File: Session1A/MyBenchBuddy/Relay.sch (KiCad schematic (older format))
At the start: 0 parts

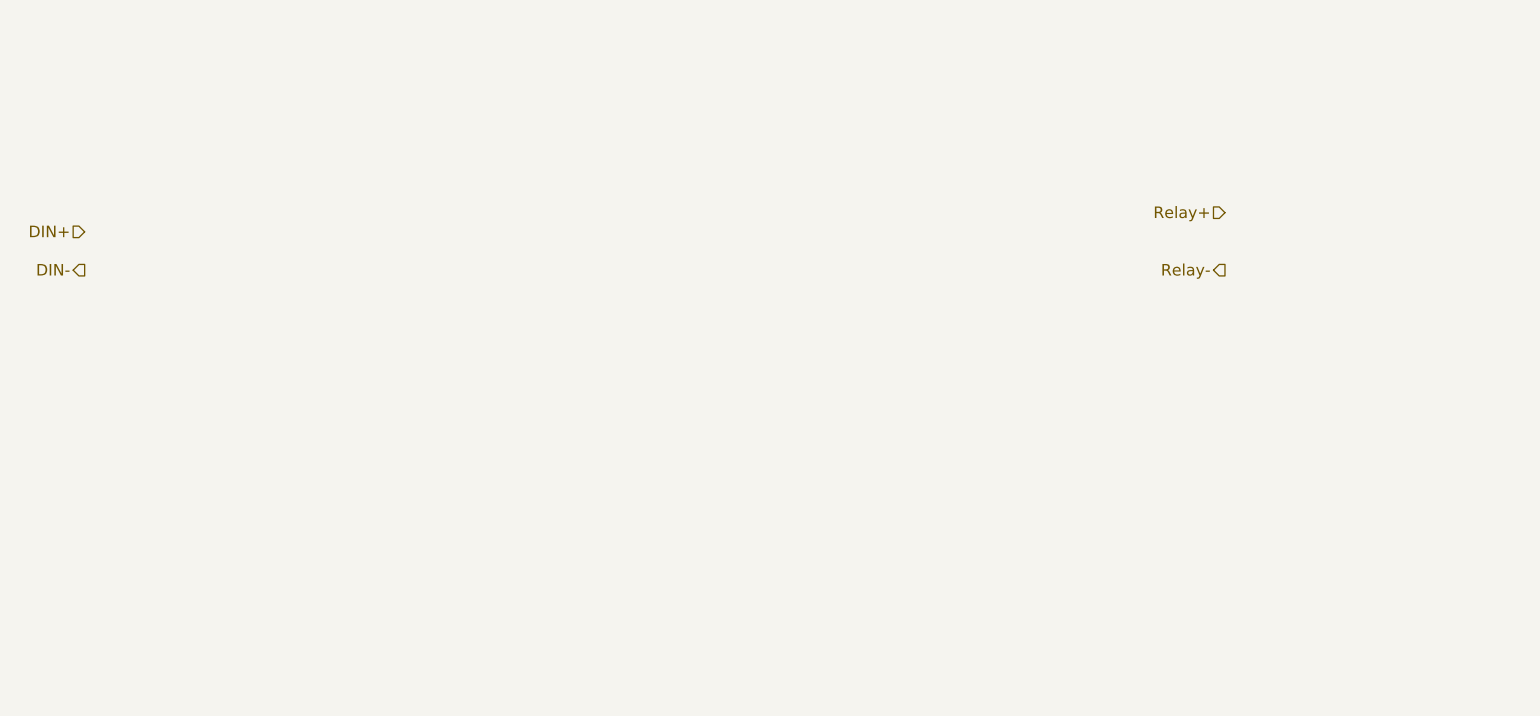
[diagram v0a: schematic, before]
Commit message: Understanding The Relay Module
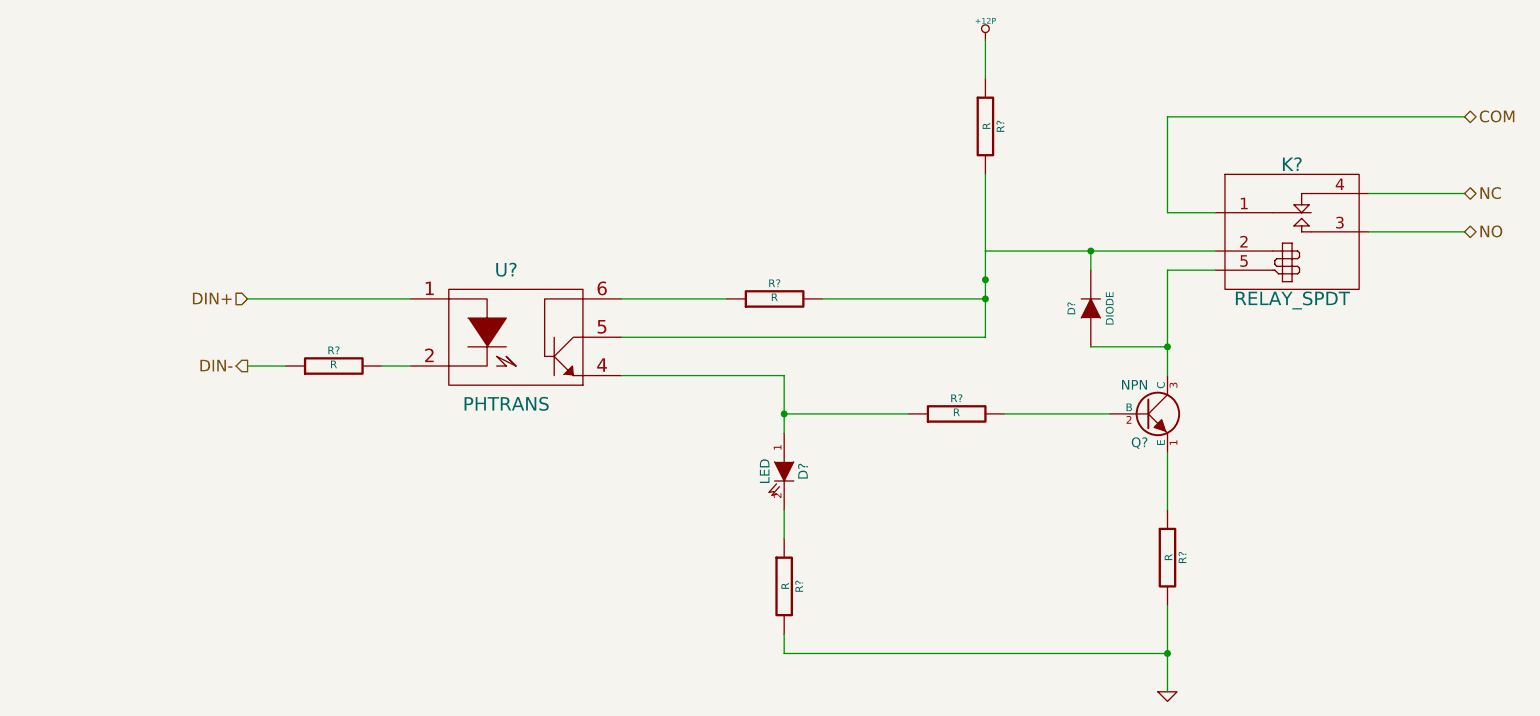
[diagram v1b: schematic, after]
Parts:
- added D?: LED, ~, symbol LED
- added D?: DIODE, ~, symbol DIODE
- added K?: RELAY_SPDT, symbol RELAY_SPDT
- added Q?: NPN, ~, symbol NPN
- added R? (x6): R, ~, symbol R
- added U?: PHTRANS, ~, symbol PHTRANS
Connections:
- net labels added: +12P, COM, GND, NC, NO
- net labels removed: Relay+, Relay-
- wire segments 0 -> 27
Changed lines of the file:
@@
 LIBS:contrib
 LIBS:valves
+LIBS:bth-switch
 LIBS:MyBenchBuddy-cache
 EELAYER 27 0
@@
 Comment4 ""
 $EndDescr
-Text HLabel 1900 2350 0    60   Input ~ 0
+Text HLabel 2750 2700 0    60   Input ~ 0
 DIN+
-Text HLabel 1900 2550 0    60   Output ~ 0
+Text HLabel 2750 3050 0    60   Output ~ 0
 DIN-
-Text HLabel 7850 2250 0    60   Input ~ 0
-Relay+
-Text HLabel 7850 2550 0    60   Output ~ 0
-Relay-
+Text HLabel 9100 2150 2    60   BiDi ~ 0
+NC
+Text HLabel 9100 2350 2    60   BiDi ~ 0
+NO
+$Comp
+L PHTRANS U?
+U 1 1 52F70E12
+P 4150 2900
+F 0 "U?" H 4100 3250 70  0000 C CNN
+F 1 "PHTRANS" H 4100 2550 70  0000 C CNN
+F 2 "~" H 4150 2900 60  0000 C CNN
+F 3 "~" H 4150 2900 60  0000 C CNN
+	1    4150 2900
+	1    0    0    -1
+$EndComp
+$Comp
+L R R?
+U 1 1 52F70E21
+P 6450 3300
+F 0 "R?" V 6530 3300 40  0000 C CNN
+F 1 "R" V 6457 3301 40  0000 C CNN
+F 2 "~" V 6380 3300 30  0000 C CNN
+F 3 "~" H 6450 3300 30  0000 C CNN
+	1    6450 3300
+	0    -1   -1   0
+$EndComp
+$Comp
+L NPN Q?
+U 1 1 52F70E30
+P 7450 3300
+F 0 "Q?" H 7450 3150 50  0000 R CNN
+F 1 "NPN" H 7450 3450 50  0000 R CNN
+F 2 "~" H 7450 3300 60  0000 C CNN
+F 3 "~" H 7450 3300 60  0000 C CNN
+	1    7450 3300
+	1    0    0    -1
+$EndComp
+$Comp
+L LED D?
+U 1 1 52F70E5D
+P 5550 3600
+F 0 "D?" H 5550 3700 50  0000 C CNN
+F 1 "LED" H 5550 3500 50  0000 C CNN
+F 2 "~" H 5550 3600 60  0000 C CNN
+F 3 "~" H 5550 3600 60  0000 C CNN
+	1    5550 3600
+	0    1    1    0
+$EndComp
+$Comp
+L RELAY_SPDT K?
+U 1 1 52F71303
+P 8200 2200
+F 0 "K?" H 8200 2400 70  0000 C CNN
+F 1 "RELAY_SPDT" H 8200 1700 70  0000 C CNN
+F 2 "" H 8200 2200 60  0000 C CNN
+F 3 "" H 8200 2200 60  0000 C CNN
+	1    8200 2200
+	1    0    0    -1
+$EndComp
+Text HLabel 9100 1750 2    60   BiDi ~ 0
+COM
+Wire Wire Line
+	9100 2150 8600 2150
+Wire Wire Line
+	9100 2350 8600 2350
+Wire Wire Line
+	6600 2450 7800 2450
+Wire Wire Line
+	6600 2050 6600 2900
+Wire Wire Line
+	7250 3300 6700 3300
+$Comp
+L R R?
+U 1 1 52F714AB
+P 7550 4050
+F 0 "R?" V 7630 4050 40  0000 C CNN
+F 1 "R" V 7557 4051 40  0000 C CNN
+F 2 "~" V 7480 4050 30  0000 C CNN
+F 3 "~" H 7550 4050 30  0000 C CNN
+	1    7550 4050
+	1    0    0    -1
+$EndComp
+Wire Wire Line
+	7550 3500 7550 3800
+$Comp
+L GND #PWR?
+U 1 1 52F715F1
+P 7550 4750
+F 0 "#PWR?" H 7550 4750 30  0001 C CNN
+F 1 "GND" H 7550 4680 30  0001 C CNN
+F 2 "" H 7550 4750 60  0000 C CNN
+F 3 "" H 7550 4750 60  0000 C CNN
+	1    7550 4750
+	1    0    0    -1
+$EndComp
+Wire Wire Line
+	7550 4300 7550 4750
+Wire Wire Line
+	5550 3300 6200 3300
+$Comp
+L R R?
+U 1 1 52F71764
+P 5550 4200
+F 0 "R?" V 5630 4200 40  0000 C CNN
+F 1 "R" V 5557 4201 40  0000 C CNN
+F 2 "~" V 5480 4200 30  0000 C CNN
+F 3 "~" H 5550 4200 30  0000 C CNN
+	1    5550 4200
+	1    0    0    -1
+$EndComp
+Wire Wire Line
+	5550 3100 5550 3400
+Connection ~ 5550 3300
+Wire Wire Line
+	5550 3800 5550 3950
+Wire Wire Line
+	5550 4450 5550 4550
+Wire Wire Line
+	5550 4550 7550 4550
+Connection ~ 7550 4550
+$Comp
+L R R?
+U 1 1 52F718DA
+P 6600 1800
+F 0 "R?" V 6680 1800 40  0000 C CNN
+F 1 "R" V 6607 1801 40  0000 C CNN
+F 2 "~" V 6530 1800 30  0000 C CNN
+F 3 "~" H 6600 1800 30  0000 C CNN
+	1    6600 1800
+	1    0    0    -1
+$EndComp
+$Comp
+L +12P #PWR?
+U 1 1 52F718E2
+P 6600 1350
+F 0 "#PWR?" H 6600 1320 30  0001 C CNN
+F 1 "+12P" H 6600 1450 30  0000 C CNN
+F 2 "" H 6600 1350 60  0000 C CNN
+F 3 "" H 6600 1350 60  0000 C CNN
+	1    6600 1350
+	1    0    0    -1
+$EndComp
+Wire Wire Line
+	6600 1350 6600 1550
+Wire Wire Line
+	6600 2900 4700 2900
+Connection ~ 6600 2600
+$Comp
+L R R?
+U 1 1 52F71E24
+P 5500 2700
+F 0 "R?" V 5580 2700 40  0000 C CNN
+F 1 "R" V 5507 2701 40  0000 C CNN
+F 2 "~" V 5430 2700 30  0000 C CNN
+F 3 "~" H 5500 2700 30  0000 C CNN
+	1    5500 2700
+	0    -1   -1   0
+$EndComp
+Wire Wire Line
+	4700 2700 5250 2700
+Wire Wire Line
+	5750 2700 6600 2700
+Connection ~ 6600 2700
+$Comp
+L R R?
+U 1 1 52F720EA
+P 3200 3050
+F 0 "R?" V 3280 3050 40  0000 C CNN
+F 1 "R" V 3207 3051 40  0000 C CNN
+F 2 "~" V 3130 3050 30  0000 C CNN
+F 3 "~" H 3200 3050 30  0000 C CNN
+	1    3200 3050
+	0    -1   -1   0
+$EndComp
+Wire Wire Line
+	2750 2700 3600 2700
+Wire Wire Line
+	3600 3050 3450 3050
+Wire Wire Line
+	2950 3050 2750 3050
+Wire Wire Line
+	7800 2250 7550 2250
+Wire Wire Line
+	7550 2250 7550 1750
+Wire Wire Line
+	7550 1750 9100 1750
+Wire Wire Line
+	7800 2550 7550 2550
+$Comp
+L DIODE D?
+U 1 1 52F726CF
+P 7150 2750
+F 0 "D?" H 7150 2850 40  0000 C CNN
+F 1 "DIODE" H 7150 2650 40  0000 C CNN
+F 2 "~" H 7150 2750 60  0000 C CNN
+F 3 "~" H 7150 2750 60  0000 C CNN
+	1    7150 2750
+	0    -1   -1   0
+$EndComp
+Wire Wire Line
+	5550 3100 4700 3100
+Wire Wire Line
+	7550 2550 7550 3100
+Wire Wire Line
+	7150 2950 7550 2950
+Connection ~ 7550 2950
+Wire Wire Line
+	7150 2550 7150 2450
+Connection ~ 7150 2450
 $EndSCHEMATC
